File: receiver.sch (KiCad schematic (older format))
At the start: 7 parts

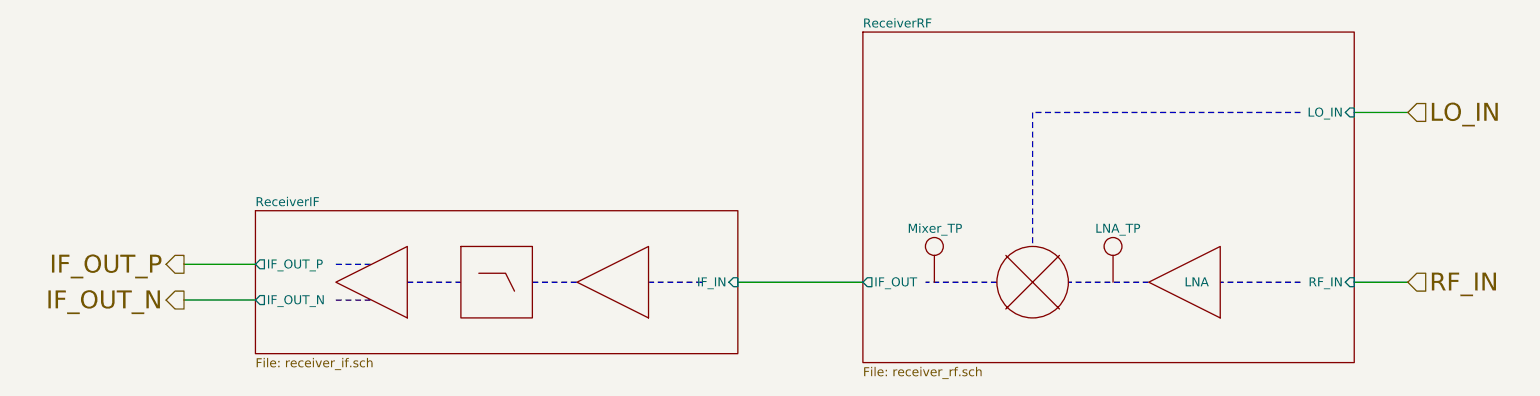
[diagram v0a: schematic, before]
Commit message: Architecture of IF
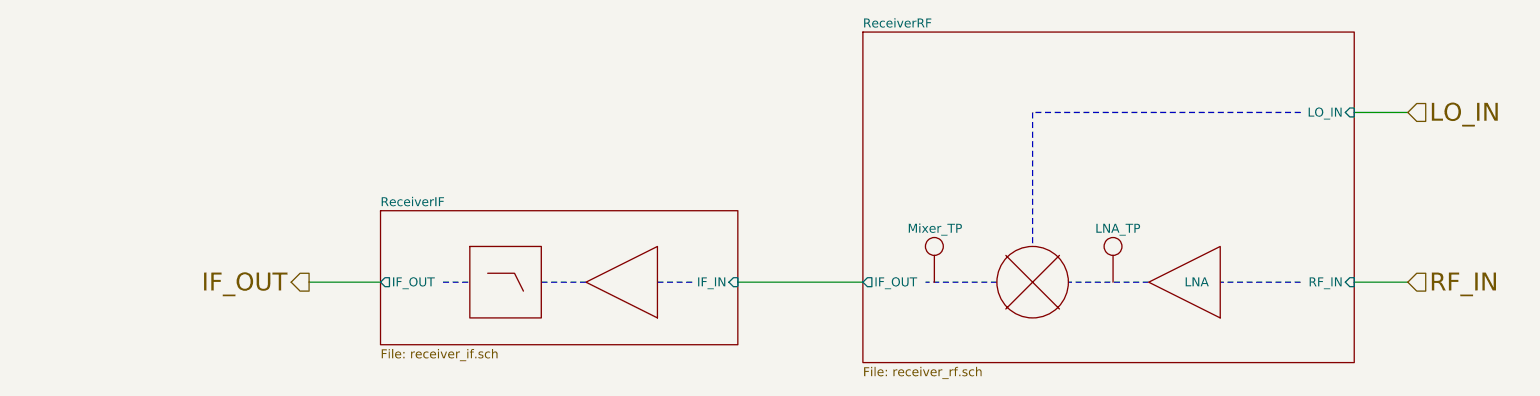
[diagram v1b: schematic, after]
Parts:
- removed U?: amplifier_diagram, symbol own:amplifier_diagram
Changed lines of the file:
@@
 $EndSheet
 $Sheet
-S 2600 3900 2700 800
+S 3300 3900 2000 750
 U 5F89D0DD
 F0 "ReceiverIF" 50
 F1 "receiver_if.sch" 50
-F2 "IF_OUT_P" O L 2600 4200 50
+F2 "IF_OUT" O L 3300 4300 50
 F3 "IF_IN" I R 5300 4300 50
-F4 "IF_OUT_N" O L 2600 4400 50
 $EndSheet
 Text HLabel 9050 3350 2    100  Input ~ 0
@@
 Wire Wire Line
 	9050 3350 8750 3350
-Text HLabel 2200 4200 0    100  Output ~ 0
-IF_OUT_P
-$Comp
-L own:amplifier_diagram U?
-U 1 1 5F89ECDE
-P 4600 4300
-F 0 "U?" H 4600 4650 50  0001 C CNN
-F 1 "amplifier_diagram" H 4372 4300 50  0001 R CNN
-F 2 "" H 4600 4300 50  0001 C CNN
-F 3 "" H 4600 4300 50  0001 C CNN
-	1    4600 4300
-	-1   0    0    1
-$EndComp
-$Comp
-L own:lowpass_diagram U?
-U 1 1 5F89F467
-P 3950 4300
-F 0 "U?" H 3950 4550 50  0001 C CNN
-F 1 "lowpass_diagram" H 3950 4050 50  0001 C CNN
-F 2 "" H 3950 4300 50  0001 C CNN
-F 3 "" H 3950 4300 50  0001 C CNN
-	1    3950 4300
-	1    0    0    -1
-$EndComp
+Text HLabel 2900 4300 0    100  Output ~ 0
+IF_OUT
 Wire Notes Line style solid rgb(132, 0, 0)
-	5100 4300 4800 4300
-$Comp
-L own:amplifier_diagram U?
-U 1 1 5F8A129E
-P 3250 4300
-F 0 "U?" H 3250 4650 50  0001 C CNN
-F 1 "amplifier_diagram" H 3022 4300 50  0001 R CNN
-F 2 "" H 3250 4300 50  0001 C CNN
-F 3 "" H 3250 4300 50  0001 C CNN
-	1    3250 4300
-	-1   0    0    1
-$EndComp
+	4450 4300 4200 4300
 Wire Notes Line style solid rgb(132, 0, 0)
-	3050 4200 3250 4200
-Wire Notes Line style solid rgb(132, 0, 0)
-	3050 4400 3250 4400
-Wire Notes Line style solid rgb(132, 0, 0)
-	3450 4300 3750 4300
-Wire Notes Line style solid rgb(132, 0, 0)
-	4150 4300 4400 4300
-Text HLabel 2200 4400 0    100  Output ~ 0
-IF_OUT_N
+	4850 4300 5050 4300
 Wire Wire Line
-	2600 4200 2200 4200
-Wire Wire Line
-	2600 4400 2200 4400
+	3300 4300 2900 4300
 Wire Wire Line
 	5300 4300 6000 4300
@@
 	1    0    0    -1
 $EndComp
+$Comp
+L own:amplifier_diagram U?
+U 1 1 5F89ECDE
+P 4650 4300
+F 0 "U?" H 4650 4650 50  0001 C CNN
+F 1 "amplifier_diagram" H 4422 4300 50  0001 R CNN
+F 2 "" H 4650 4300 50  0001 C CNN
+F 3 "" H 4650 4300 50  0001 C CNN
+	1    4650 4300
+	-1   0    0    1
+$EndComp
+$Comp
+L own:lowpass_diagram U?
+U 1 1 5F89F467
+P 4000 4300
+F 0 "U?" H 4000 4550 50  0001 C CNN
+F 1 "lowpass_diagram" H 4000 4050 50  0001 C CNN
+F 2 "" H 4000 4300 50  0001 C CNN
+F 3 "" H 4000 4300 50  0001 C CNN
+	1    4000 4300
+	1    0    0    -1
+$EndComp
+Wire Notes Line style solid rgb(132, 0, 0)
+	3650 4300 3800 4300
 $EndSCHEMATC
